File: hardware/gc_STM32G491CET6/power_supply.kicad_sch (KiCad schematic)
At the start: 20 parts, among them U6 AZ1117CH2-5.0TRG1, U7 MIC5317-3.3YM5-TR

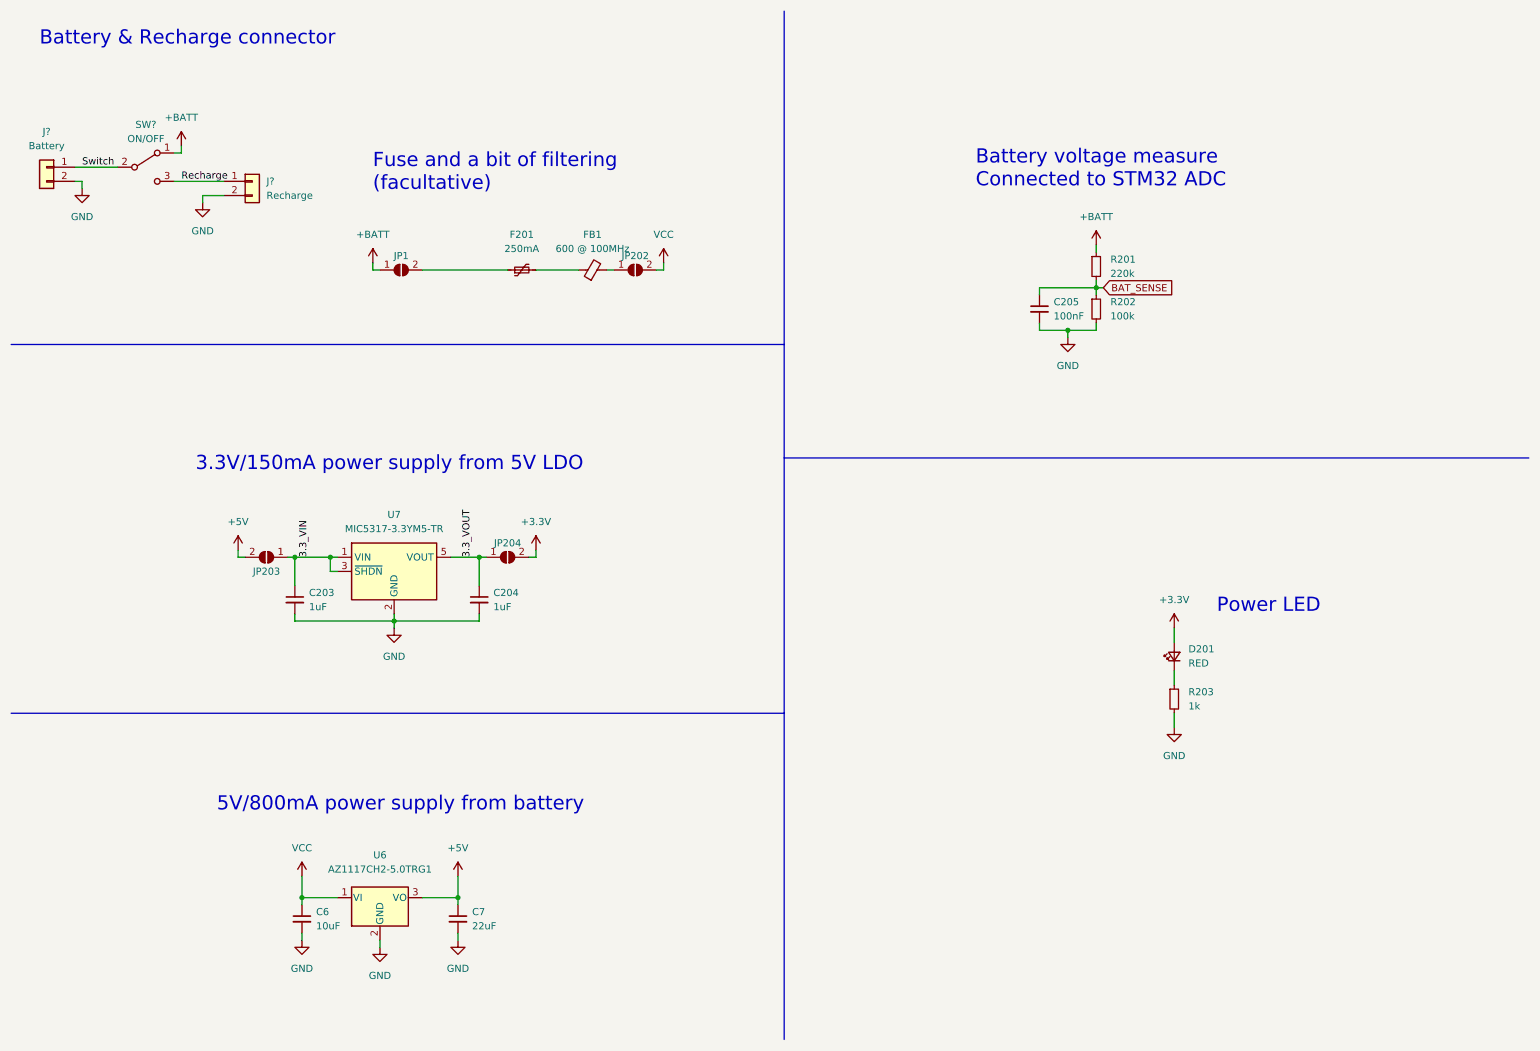
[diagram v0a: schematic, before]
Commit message: Schematics + rough placement
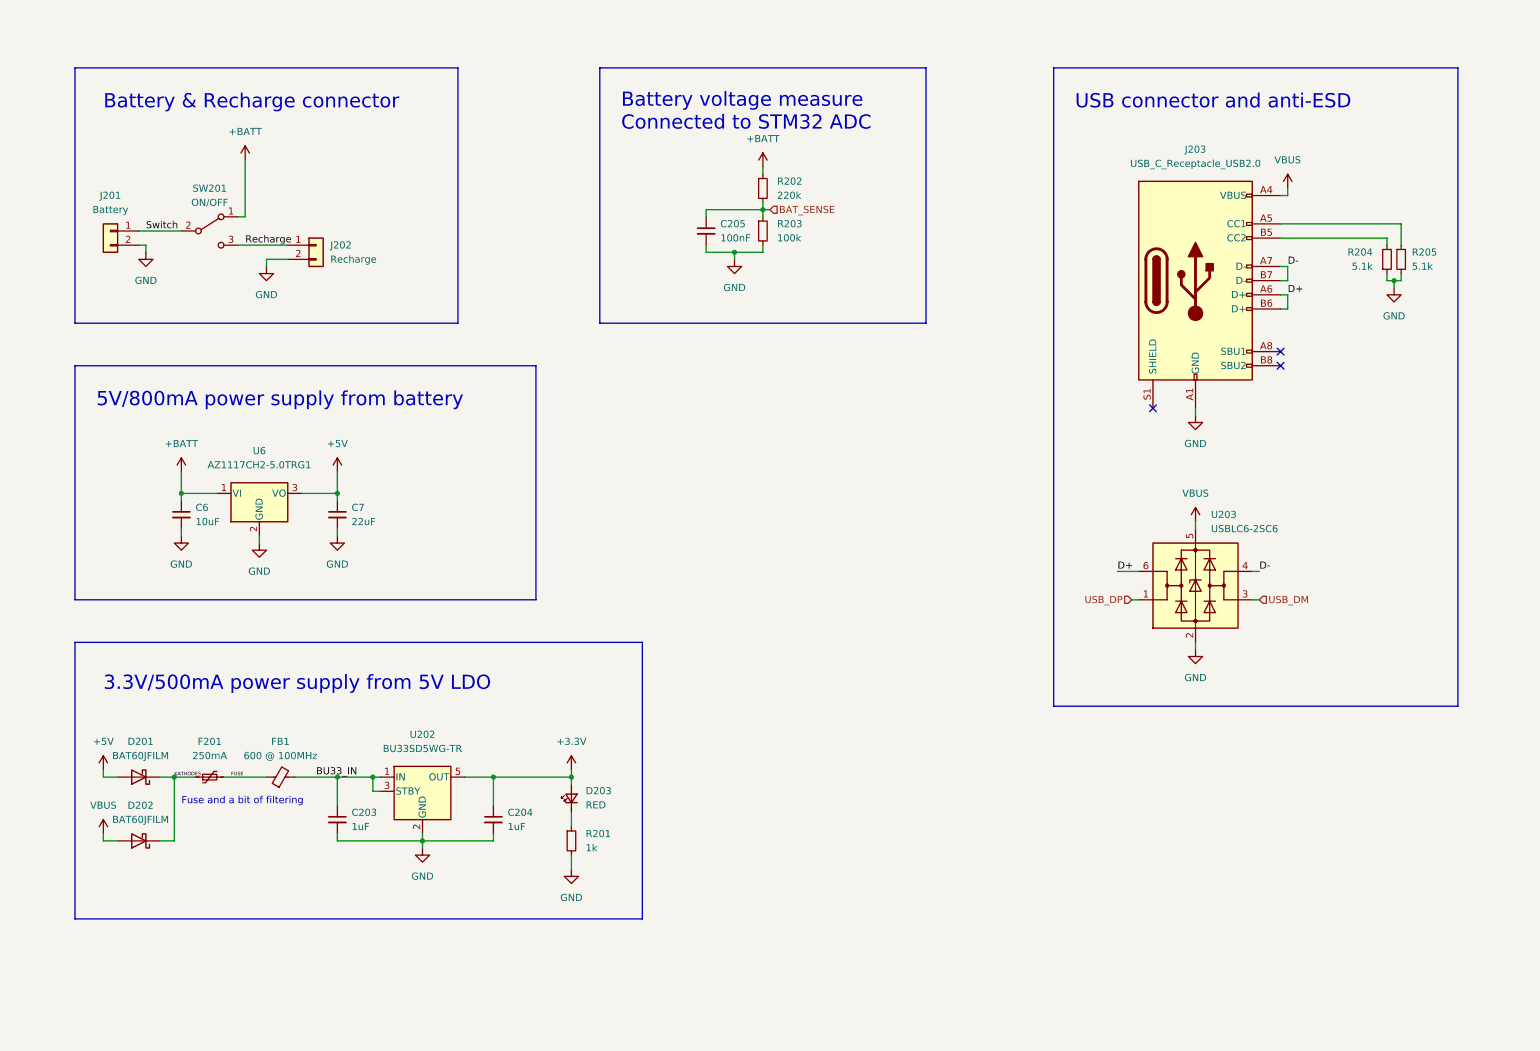
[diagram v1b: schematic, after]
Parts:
- removed JP1, JP202, JP203, JP204: SolderJumper_2_Open, Jumper:SolderJumper-2_P1.3mm_Open_TrianglePad1.0x1.5mm, symbol Jumper:SolderJumper_2_Open
- removed U7: MIC5317-3.3YM5-TR, Package_TO_SOT_SMD:SOT-23-5, symbol Regulator_Linear:MCP1802x-xx02xOT
- added D201, D202: BAT60JFILM, Diode_SMD:D_SOD-323, symbol Diode:BAT60A
- added J203: USB_C_Receptacle_USB2.0, Connector_USB:USB_C_Receptacle_HRO_TYPE-C-31-M-12, symbol Connector:USB_C_Receptacle_USB2.0
- added R204, R205: 5.1k, Resistor_SMD:R_0603_1608Metric_Pad0.98x0.95mm_HandSolder, symbol Device:R_Small
- added U202: BU33SD5WG-TR, Package_TO_SOT_SMD:SOT-23-5, symbol WITNS_ROHM:BU33SD5WG-TR
- added U203: USBLC6-2SC6, Package_TO_SOT_SMD:SOT-23-6, symbol Power_Protection:USBLC6-2SC6
- SW201: renamed from SW?; footprint RS_switch:RS_Switch_448-0747 -> WITNS:RS_Switch_448-0747
- gave numbers to parts that had none: 2
- renumbered D201 to D203, R203 to R201, R201 to R202, R202 to R203
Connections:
- net 3.3_VIN is gone; now on net BU33_IN: C203.1
- net 3.3_VOUT is gone; now on net +3.3V: C204.1
- net VCC is gone; now on net +BATT: C6.1, U6.1 (VI)
- net +5V: now also D201.2 (A)
- net GND: now also J203.A1 (GND), J203.A12 (GND), J203.B1 (GND), J203.B12 (GND), R204.1, R205.2, U202.2 (GND), U203.2 (GND)
- net FUSE: now reaches F201.2, FB1.1
- net BU33_IN: now reaches FB1.2
- net BU33_IN: now also U202.1 (IN), U202.3 (STBY)
- net KATHODES: now reaches F201.1
- net KATHODES: now also D201.1 (K), D202.1 (K)
- net +3V3 renamed +3.3V
- net +3.3V: now also U202.5 (OUT)
- new net: J203.B5 (CC2), R204.2
- new net: J203.A5 (CC1), R205.1
- new net D+: J203.A6 (D+), J203.B6 (D+), U203.6 (I/O1)
- new net D-: J203.A7 (D-), J203.B7 (D-), U203.4 (I/O2)
- new net USB_DM: U203.3 (I/O2)
- new net USB_DP: U203.1 (I/O1)
- new net VBUS: D202.2 (A), J203.A4 (VBUS), J203.A9 (VBUS), J203.B4 (VBUS), J203.B9 (VBUS), U203.5 (VBUS)
- no-connect marks 0 -> 3
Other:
- note added: "3.3V/500mA power supply from 5V LDO"
- note added: "Fuse and a bit of filtering"
- note added: "USB connector and anti-ESD"
- note removed: "3.3V/150mA power supply from 5V LDO"
- note removed: "Fuse and a bit of filtering (facultative)"
- note removed: "Power LED"
- moved on the sheet: C203, C204, C205, C6, C7, D203, J201, J202, R201, R202, R203, SW201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

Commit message: placement
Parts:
- C203, C204, C205: footprint Capacitor_SMD:C_0603_1608Metric_Pad1.08x0.95mm_HandSolder -> Capacitor_SMD:C_0603_1608Metric
- D203: footprint LED_SMD:LED_0603_1608Metric_Pad1.05x0.95mm_HandSolder -> LED_SMD:LED_0603_1608Metric
- R201, R202, R203, R204, R205: footprint Resistor_SMD:R_0603_1608Metric_Pad0.98x0.95mm_HandSolder -> Resistor_SMD:R_0603_1608Metric
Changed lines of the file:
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@@
       (effects (font (size 1.27 1.27)) (justify left))
     )
-    (property "Footprint" "Capacitor_SMD:C_0603_1608Metric_Pad1.08x0.95mm_HandSolder" (id 2) (at 43.18 102.87 0)
+    (property "Footprint" "Capacitor_SMD:C_0603_1608Metric" (id 2) (at 43.18 102.87 0)
       (effects (font (size 1.27 1.27)) hide)
     )
@@
       (effects (font (size 1.27 1.27)) (justify left))
     )
-    (property "Footprint" "Capacitor_SMD:C_0603_1608Metric_Pad1.08x0.95mm_HandSolder" (id 2) (at 99.06 157.48 0)
+    (property "Footprint" "Capacitor_SMD:C_0603_1608Metric" (id 2) (at 99.06 157.48 0)
       (effects (font (size 1.27 1.27)) hide)
     )
@@
       (effects (font (size 1.27 1.27)) (justify right))
     )
-    (property "Footprint" "Resistor_SMD:R_0603_1608Metric_Pad0.98x0.95mm_HandSolder" (id 2) (at 259.08 57.15 0)
+    (property "Footprint" "Resistor_SMD:R_0603_1608Metric" (id 2) (at 259.08 57.15 0)
       (effects (font (size 1.27 1.27)) hide)
     )
@@
       (effects (font (size 1.27 1.27)) (justify left))
     )
-    (property "Footprint" "Capacitor_SMD:C_0603_1608Metric_Pad1.08x0.95mm_HandSolder" (id 2) (at 71.12 157.48 0)
+    (property "Footprint" "Capacitor_SMD:C_0603_1608Metric" (id 2) (at 71.12 157.48 0)
       (effects (font (size 1.27 1.27)) hide)
     )
@@
       (effects (font (size 1.27 1.27)) (justify left))
     )
-    (property "Footprint" "Resistor_SMD:R_0603_1608Metric_Pad0.98x0.95mm_HandSolder" (id 2) (at 147.32 44.45 0)
+    (property "Footprint" "Resistor_SMD:R_0603_1608Metric" (id 2) (at 147.32 44.45 0)
       (effects (font (size 1.27 1.27)) hide)
     )
@@
       (effects (font (size 1.27 1.27)) (justify left))
     )
-    (property "Footprint" "Capacitor_SMD:C_0603_1608Metric_Pad1.08x0.95mm_HandSolder" (id 2) (at 71.12 102.87 0)
+    (property "Footprint" "Capacitor_SMD:C_0603_1608Metric" (id 2) (at 71.12 102.87 0)
       (effects (font (size 1.27 1.27)) hide)
     )
@@
       (effects (font (size 1.27 1.27)) (justify left))
     )
-    (property "Footprint" "Resistor_SMD:R_0603_1608Metric_Pad0.98x0.95mm_HandSolder" (id 2) (at 147.32 52.07 0)
+    (property "Footprint" "Resistor_SMD:R_0603_1608Metric" (id 2) (at 147.32 52.07 0)
       (effects (font (size 1.27 1.27)) hide)
     )
@@
       (effects (font (size 1.27 1.27)) (justify right))
     )
-    (property "Footprint" "LED_SMD:LED_0603_1608Metric_Pad1.05x0.95mm_HandSolder" (id 2) (at 113.03 153.67 90)
+    (property "Footprint" "LED_SMD:LED_0603_1608Metric" (id 2) (at 113.03 153.67 90)
       (effects (font (size 1.27 1.27)) hide)
     )
@@
       (effects (font (size 1.27 1.27)) (justify left))
     )
-    (property "Footprint" "Resistor_SMD:R_0603_1608Metric_Pad0.98x0.95mm_HandSolder" (id 2) (at 261.62 57.15 0)
+    (property "Footprint" "Resistor_SMD:R_0603_1608Metric" (id 2) (at 261.62 57.15 0)
       (effects (font (size 1.27 1.27)) hide)
     )
@@
     (property "Reference" "FB201" (id 0) (at 60.9219 143.51 90))
     (property "Value" "600 @ 100MHz" (id 1) (at 60.9219 146.05 90))
-    (property "Footprint" "Inductor_SMD:L_0805_2012Metric_Pad1.05x1.20mm_HandSolder" (id 2) (at 60.96 151.638 90)
+    (property "Footprint" "Inductor_SMD:L_0805_2012Metric" (id 2) (at 60.96 151.638 90)
       (effects (font (size 1.27 1.27)) hide)
     )
@@
       (effects (font (size 1.27 1.27)) (justify left))
     )
-    (property "Footprint" "Capacitor_SMD:C_0603_1608Metric_Pad1.08x0.95mm_HandSolder" (id 2) (at 137.16 52.07 0)
+    (property "Footprint" "Capacitor_SMD:C_0603_1608Metric" (id 2) (at 137.16 52.07 0)
       (effects (font (size 1.27 1.27)) hide)
     )
@@
       (effects (font (size 1.27 1.27)) (justify left))
     )
-    (property "Footprint" "Resistor_SMD:R_0603_1608Metric_Pad0.98x0.95mm_HandSolder" (id 2) (at 113.03 161.29 0)
-      (effects (font (size 1.27 1.27)) hide)
-    )
+    (property "Footprint" "Resistor_SMD:R_0603_1608Metric" (id 2) (at 113.03 161.29 0)
+      (effects (font (size 1.27 1.27)) hide)
+    )
